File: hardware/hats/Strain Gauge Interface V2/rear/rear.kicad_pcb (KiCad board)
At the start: 2 copper layers, 78 x 58 mm, 76 parts, among them J1 Conn_01x14, U1 ADS1235IRHBT, U2 ADS1235IRHBT, U3 LMR50410YQDBVRQ1, U5 BD450, U6 BD433

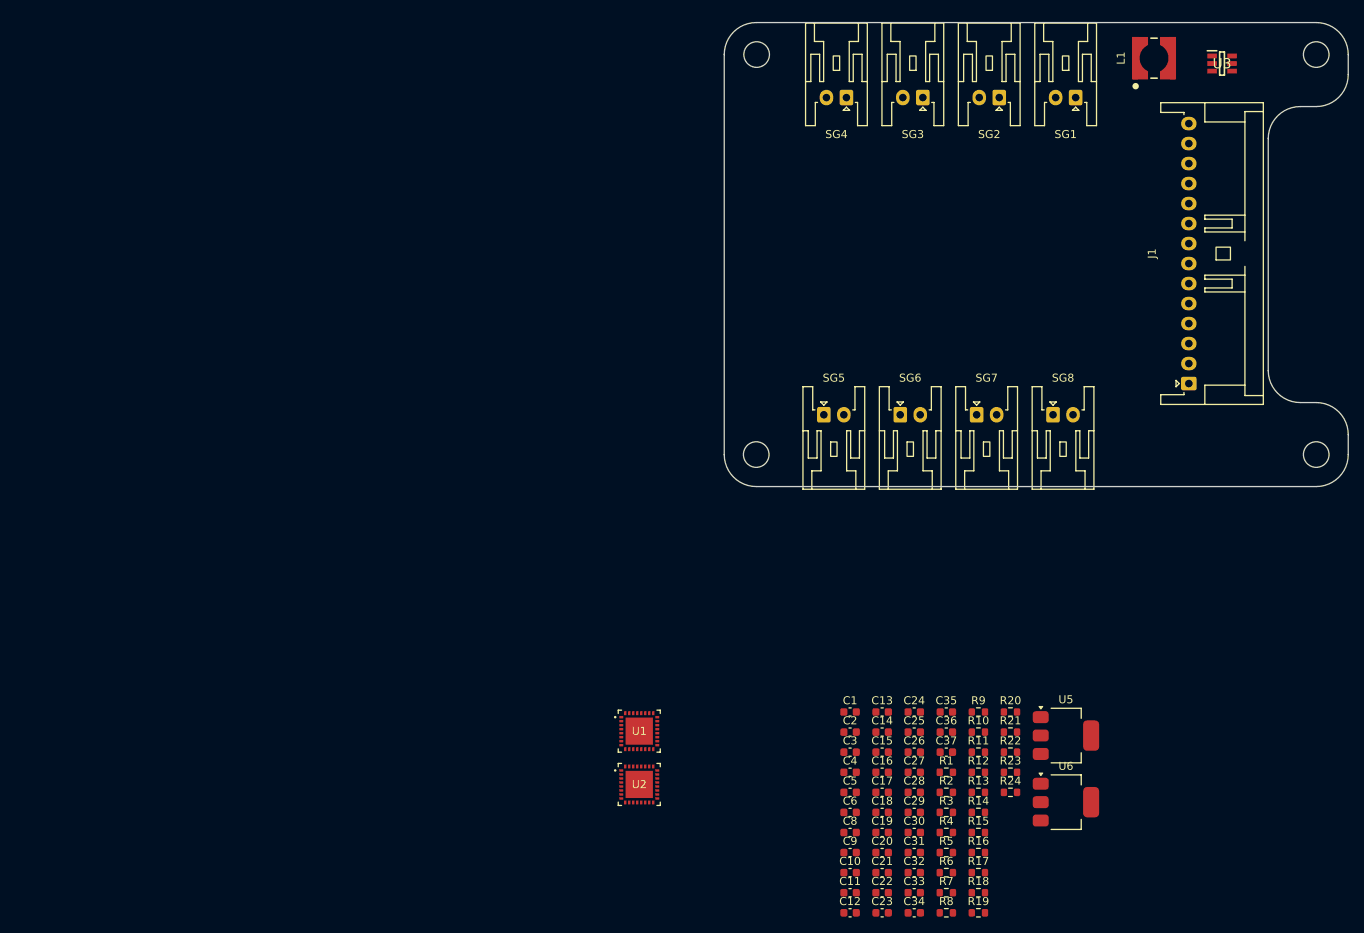
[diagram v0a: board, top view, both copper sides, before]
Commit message: this is worse than torture
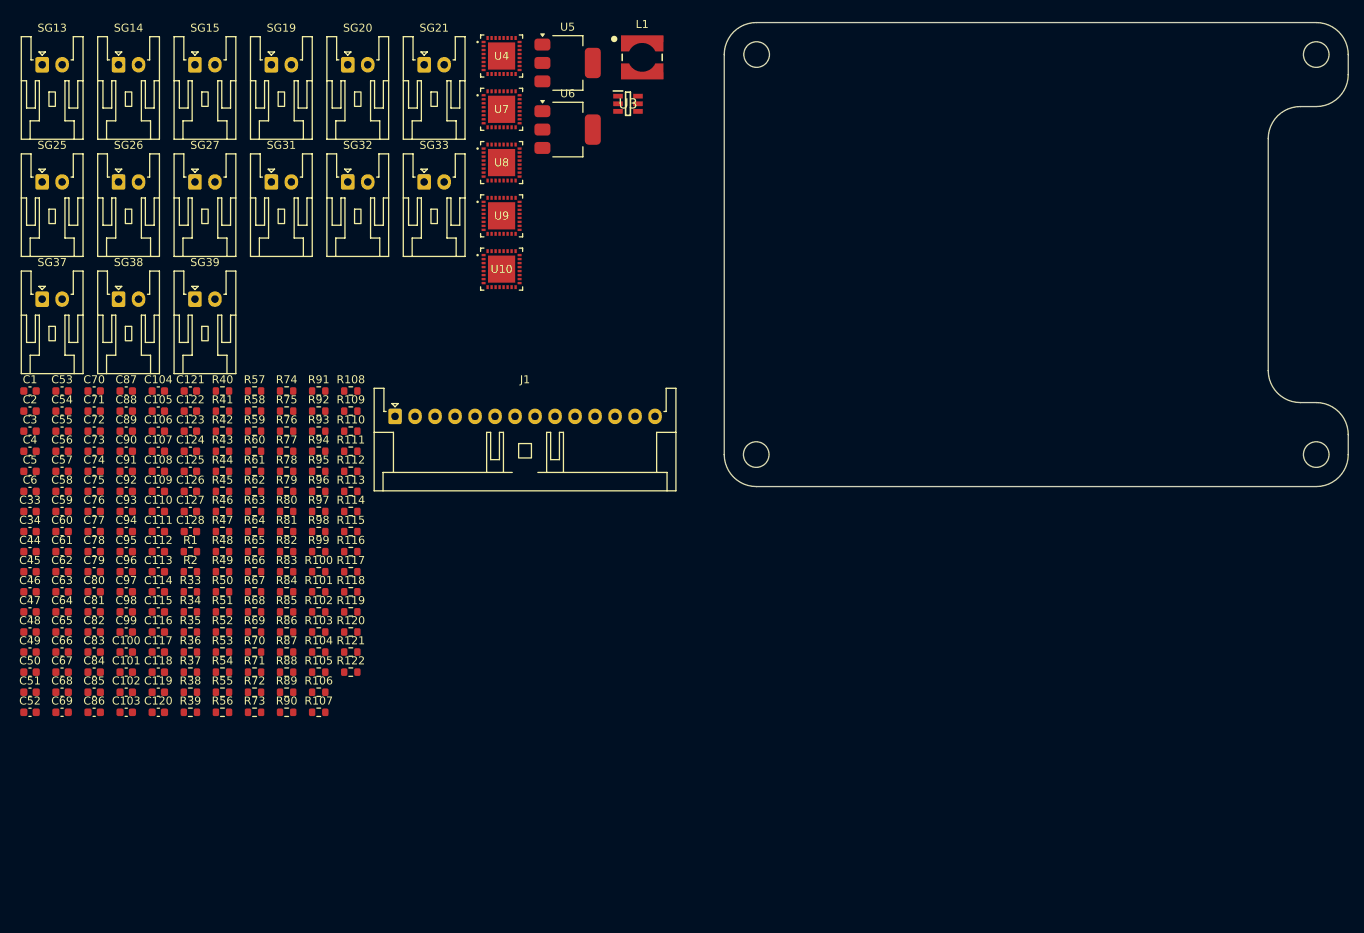
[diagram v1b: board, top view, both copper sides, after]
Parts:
- removed C10, C11, C12, C13, C14, C15, C17, C8: 1uf, Capacitor_SMD:C_0603_1608Metric
- removed C16, C18, C21, C26, C29, C32, C37, C9: 10nf, Capacitor_SMD:C_0603_1608Metric
- removed C19, C20, C22, C23, C24, C25, C27, C28, C30, C31, C35, C36: 1nf, Capacitor_SMD:C_0603_1608Metric
- removed R10, R11, R14, R15, R18, R19, R23, R24, R6, R7, R8, R9: 100, Resistor_SMD:R_0603_1608Metric
- removed R12, R13, R16, R17, R20, R21, R3, R5: 120, Resistor_SMD:R_0603_1608Metric
- removed R22, R4: 100k, Resistor_SMD:R_0603_1608Metric
- removed SG1, SG3, SG5, SG7: TOP, Connector_JST:JST_XA_S02B-XASK-1_1x02_P2.50mm_Horizontal
- removed SG2, SG4, SG6, SG8: BOTTOM, Connector_JST:JST_XA_S02B-XASK-1_1x02_P2.50mm_Horizontal
- removed U1, U2: ADS1235IRHBT, CustomFootprints:RHB32_TEX
- added C100: 1nf, Capacitor_SMD:C_0603_1608Metric, F.Cu at (32.2, 136.1)
- added C101: 10nf, Capacitor_SMD:C_0603_1608Metric, F.Cu at (32.2, 138.6)
- added C102: 10nf, Capacitor_SMD:C_0603_1608Metric, F.Cu at (32.2, 141.1)
- added C103: 10nf, Capacitor_SMD:C_0603_1608Metric, F.Cu at (32.2, 143.6)
- added C104: 1nf, Capacitor_SMD:C_0603_1608Metric, F.Cu at (36.3, 103.4)
- added C105: 1nf, Capacitor_SMD:C_0603_1608Metric, F.Cu at (36.3, 105.9)
- added C106: 1nf, Capacitor_SMD:C_0603_1608Metric, F.Cu at (36.3, 108.5)
- added C107: 1nf, Capacitor_SMD:C_0603_1608Metric, F.Cu at (36.3, 111.0)
- added C108: 1nf, Capacitor_SMD:C_0603_1608Metric, F.Cu at (36.3, 113.5)
- added C109: 1nf, Capacitor_SMD:C_0603_1608Metric, F.Cu at (36.3, 116.0)
- added C110: 10nf, Capacitor_SMD:C_0603_1608Metric, F.Cu at (36.3, 118.5)
- added C111: 10nf, Capacitor_SMD:C_0603_1608Metric, F.Cu at (36.3, 121.0)
- added C112: 10nf, Capacitor_SMD:C_0603_1608Metric, F.Cu at (36.3, 123.5)
- added C113: 1uf, Capacitor_SMD:C_0603_1608Metric, F.Cu at (36.3, 126.0)
- added C114: 1uf, Capacitor_SMD:C_0603_1608Metric, F.Cu at (36.3, 128.5)
- added C115: 1uf, Capacitor_SMD:C_0603_1608Metric, F.Cu at (36.3, 131.0)
- added C116: 10nf, Capacitor_SMD:C_0603_1608Metric, F.Cu at (36.3, 133.6)
- added C117: 1uf, Capacitor_SMD:C_0603_1608Metric, F.Cu at (36.3, 136.1)
- added C118: 1nf, Capacitor_SMD:C_0603_1608Metric, F.Cu at (36.3, 138.6)
- added C119: 1nf, Capacitor_SMD:C_0603_1608Metric, F.Cu at (36.3, 141.1)
- added C120: 10nf, Capacitor_SMD:C_0603_1608Metric, F.Cu at (36.3, 143.6)
- added C121: 1uf, Capacitor_SMD:C_0603_1608Metric, F.Cu at (40.3, 103.4)
- added C122: 1uf, Capacitor_SMD:C_0603_1608Metric, F.Cu at (40.3, 105.9)
- added C123: 1uf, Capacitor_SMD:C_0603_1608Metric, F.Cu at (40.3, 108.5)
- added C124: 10nf, Capacitor_SMD:C_0603_1608Metric, F.Cu at (40.3, 111.0)
- added C125: 1uf, Capacitor_SMD:C_0603_1608Metric, F.Cu at (40.3, 113.5)
- added C126: 1nf, Capacitor_SMD:C_0603_1608Metric, F.Cu at (40.3, 116.0)
- added C127: 1nf, Capacitor_SMD:C_0603_1608Metric, F.Cu at (40.3, 118.5)
- added C128: 10nf, Capacitor_SMD:C_0603_1608Metric, F.Cu at (40.3, 121.0)
- added C44: 1uf, Capacitor_SMD:C_0603_1608Metric, F.Cu at (20.2, 123.5)
- added C45: 1uf, Capacitor_SMD:C_0603_1608Metric, F.Cu at (20.2, 126.0)
- added C46: 1uf, Capacitor_SMD:C_0603_1608Metric, F.Cu at (20.2, 128.5)
- added C47: 1uf, Capacitor_SMD:C_0603_1608Metric, F.Cu at (20.2, 131.0)
- added C48: 1uf, Capacitor_SMD:C_0603_1608Metric, F.Cu at (20.2, 133.6)
- added C49: 1uf, Capacitor_SMD:C_0603_1608Metric, F.Cu at (20.2, 136.1)
- added C50: 10nf, Capacitor_SMD:C_0603_1608Metric, F.Cu at (20.2, 138.6)
- added C51: 10nf, Capacitor_SMD:C_0603_1608Metric, F.Cu at (20.2, 141.1)
- added C52: 1uf, Capacitor_SMD:C_0603_1608Metric, F.Cu at (20.2, 143.6)
- added C53: 1uf, Capacitor_SMD:C_0603_1608Metric, F.Cu at (24.2, 103.4)
- added C54: 1nf, Capacitor_SMD:C_0603_1608Metric, F.Cu at (24.2, 105.9)
- added C55: 1nf, Capacitor_SMD:C_0603_1608Metric, F.Cu at (24.2, 108.5)
- added C56: 1nf, Capacitor_SMD:C_0603_1608Metric, F.Cu at (24.2, 111.0)
- added C57: 1nf, Capacitor_SMD:C_0603_1608Metric, F.Cu at (24.2, 113.5)
- added C58: 10nf, Capacitor_SMD:C_0603_1608Metric, F.Cu at (24.2, 116.0)
- added C59: 10nf, Capacitor_SMD:C_0603_1608Metric, F.Cu at (24.2, 118.5)
- added C60: 1uf, Capacitor_SMD:C_0603_1608Metric, F.Cu at (24.2, 121.0)
- added C61: 1uf, Capacitor_SMD:C_0603_1608Metric, F.Cu at (24.2, 123.5)
- added C62: 1uf, Capacitor_SMD:C_0603_1608Metric, F.Cu at (24.2, 126.0)
- added C63: 10nf, Capacitor_SMD:C_0603_1608Metric, F.Cu at (24.2, 128.5)
- added C64: 1uf, Capacitor_SMD:C_0603_1608Metric, F.Cu at (24.2, 131.0)
- added C65: 1nf, Capacitor_SMD:C_0603_1608Metric, F.Cu at (24.2, 133.6)
- added C66: 1nf, Capacitor_SMD:C_0603_1608Metric, F.Cu at (24.2, 136.1)
- added C67: 10nf, Capacitor_SMD:C_0603_1608Metric, F.Cu at (24.2, 138.6)
- added C68: 1nf, Capacitor_SMD:C_0603_1608Metric, F.Cu at (24.2, 141.1)
- added C69: 1nf, Capacitor_SMD:C_0603_1608Metric, F.Cu at (24.2, 143.6)
- added C70: 1nf, Capacitor_SMD:C_0603_1608Metric, F.Cu at (28.2, 103.4)
- added C71: 1nf, Capacitor_SMD:C_0603_1608Metric, F.Cu at (28.2, 105.9)
- added C72: 1nf, Capacitor_SMD:C_0603_1608Metric, F.Cu at (28.2, 108.5)
- added C73: 1nf, Capacitor_SMD:C_0603_1608Metric, F.Cu at (28.2, 111.0)
- added C74: 10nf, Capacitor_SMD:C_0603_1608Metric, F.Cu at (28.2, 113.5)
- added C75: 10nf, Capacitor_SMD:C_0603_1608Metric, F.Cu at (28.2, 116.0)
- added C76: 10nf, Capacitor_SMD:C_0603_1608Metric, F.Cu at (28.2, 118.5)
- added C77: 1nf, Capacitor_SMD:C_0603_1608Metric, F.Cu at (28.2, 121.0)
- added C78: 1nf, Capacitor_SMD:C_0603_1608Metric, F.Cu at (28.2, 123.5)
- added C79: 1nf, Capacitor_SMD:C_0603_1608Metric, F.Cu at (28.2, 126.0)
- added C80: 1nf, Capacitor_SMD:C_0603_1608Metric, F.Cu at (28.2, 128.5)
- added C81: 1nf, Capacitor_SMD:C_0603_1608Metric, F.Cu at (28.2, 131.0)
- added C82: 1nf, Capacitor_SMD:C_0603_1608Metric, F.Cu at (28.2, 133.6)
- added C83: 10nf, Capacitor_SMD:C_0603_1608Metric, F.Cu at (28.2, 136.1)
- added C84: 10nf, Capacitor_SMD:C_0603_1608Metric, F.Cu at (28.2, 138.6)
- added C85: 10nf, Capacitor_SMD:C_0603_1608Metric, F.Cu at (28.2, 141.1)
- added C86: 1nf, Capacitor_SMD:C_0603_1608Metric, F.Cu at (28.2, 143.6)
- added C87: 1nf, Capacitor_SMD:C_0603_1608Metric, F.Cu at (32.2, 103.4)
- added C88: 1nf, Capacitor_SMD:C_0603_1608Metric, F.Cu at (32.2, 105.9)
- added C89: 1nf, Capacitor_SMD:C_0603_1608Metric, F.Cu at (32.2, 108.5)
- added C90: 1nf, Capacitor_SMD:C_0603_1608Metric, F.Cu at (32.2, 111.0)
- added C91: 1nf, Capacitor_SMD:C_0603_1608Metric, F.Cu at (32.2, 113.5)
- added C92: 10nf, Capacitor_SMD:C_0603_1608Metric, F.Cu at (32.2, 116.0)
- added C93: 10nf, Capacitor_SMD:C_0603_1608Metric, F.Cu at (32.2, 118.5)
- added C94: 10nf, Capacitor_SMD:C_0603_1608Metric, F.Cu at (32.2, 121.0)
- added C95: 1nf, Capacitor_SMD:C_0603_1608Metric, F.Cu at (32.2, 123.5)
- added C96: 1nf, Capacitor_SMD:C_0603_1608Metric, F.Cu at (32.2, 126.0)
- added C97: 1nf, Capacitor_SMD:C_0603_1608Metric, F.Cu at (32.2, 128.5)
- added C98: 1nf, Capacitor_SMD:C_0603_1608Metric, F.Cu at (32.2, 131.0)
- added C99: 1nf, Capacitor_SMD:C_0603_1608Metric, F.Cu at (32.2, 133.6)
- added R100: 120, Resistor_SMD:R_0603_1608Metric, F.Cu at (56.3, 126.0)
- added R101: 120, Resistor_SMD:R_0603_1608Metric, F.Cu at (56.3, 128.5)
- added R102: 120, Resistor_SMD:R_0603_1608Metric, F.Cu at (56.3, 131.0)
- added R103: 120, Resistor_SMD:R_0603_1608Metric, F.Cu at (56.3, 133.6)
- added R104: 120, Resistor_SMD:R_0603_1608Metric, F.Cu at (56.3, 136.1)
- added R105: 120, Resistor_SMD:R_0603_1608Metric, F.Cu at (56.3, 138.6)
- added R106: 120, Resistor_SMD:R_0603_1608Metric, F.Cu at (56.3, 141.1)
- added R107: 120, Resistor_SMD:R_0603_1608Metric, F.Cu at (56.3, 143.6)
- added R108: 120, Resistor_SMD:R_0603_1608Metric, F.Cu at (60.3, 103.4)
- added R109: 120, Resistor_SMD:R_0603_1608Metric, F.Cu at (60.3, 105.9)
- added R110: 120, Resistor_SMD:R_0603_1608Metric, F.Cu at (60.3, 108.5)
- added R111: 120, Resistor_SMD:R_0603_1608Metric, F.Cu at (60.3, 111.0)
- added R112: 120, Resistor_SMD:R_0603_1608Metric, F.Cu at (60.3, 113.5)
- added R113: 120, Resistor_SMD:R_0603_1608Metric, F.Cu at (60.3, 116.0)
- added R114: 120, Resistor_SMD:R_0603_1608Metric, F.Cu at (60.3, 118.5)
- added R115: 120, Resistor_SMD:R_0603_1608Metric, F.Cu at (60.3, 121.0)
- added R116: 120, Resistor_SMD:R_0603_1608Metric, F.Cu at (60.3, 123.5)
- added R117: 100k, Resistor_SMD:R_0603_1608Metric, F.Cu at (60.3, 126.0)
- added R118: 100, Resistor_SMD:R_0603_1608Metric, F.Cu at (60.3, 128.5)
- added R119: 100, Resistor_SMD:R_0603_1608Metric, F.Cu at (60.3, 131.0)
- added R120: 100k, Resistor_SMD:R_0603_1608Metric, F.Cu at (60.3, 133.6)
- added R121: 100, Resistor_SMD:R_0603_1608Metric, F.Cu at (60.3, 136.1)
- added R122: 100, Resistor_SMD:R_0603_1608Metric, F.Cu at (60.3, 138.6)
- added R33: 100k, Resistor_SMD:R_0603_1608Metric, F.Cu at (40.3, 128.5)
- added R34: 100k, Resistor_SMD:R_0603_1608Metric, F.Cu at (40.3, 131.0)
- added R35: 100, Resistor_SMD:R_0603_1608Metric, F.Cu at (40.3, 133.6)
- added R36: 100, Resistor_SMD:R_0603_1608Metric, F.Cu at (40.3, 136.1)
- added R37: 100, Resistor_SMD:R_0603_1608Metric, F.Cu at (40.3, 138.6)
- added R38: 100, Resistor_SMD:R_0603_1608Metric, F.Cu at (40.3, 141.1)
- added R39: 100k, Resistor_SMD:R_0603_1608Metric, F.Cu at (40.3, 143.6)
- added R40: 100, Resistor_SMD:R_0603_1608Metric, F.Cu at (44.3, 103.4)
- added R41: 100, Resistor_SMD:R_0603_1608Metric, F.Cu at (44.3, 105.9)
- added R42: 100, Resistor_SMD:R_0603_1608Metric, F.Cu at (44.3, 108.5)
- added R43: 100, Resistor_SMD:R_0603_1608Metric, F.Cu at (44.3, 111.0)
- added R44: 100, Resistor_SMD:R_0603_1608Metric, F.Cu at (44.3, 113.5)
- added R45: 100, Resistor_SMD:R_0603_1608Metric, F.Cu at (44.3, 116.0)
- added R46: 100, Resistor_SMD:R_0603_1608Metric, F.Cu at (44.3, 118.5)
- added R47: 100, Resistor_SMD:R_0603_1608Metric, F.Cu at (44.3, 121.0)
- added R48: 120, Resistor_SMD:R_0603_1608Metric, F.Cu at (44.3, 123.5)
- added R49: 120, Resistor_SMD:R_0603_1608Metric, F.Cu at (44.3, 126.0)
- added R50: 120, Resistor_SMD:R_0603_1608Metric, F.Cu at (44.3, 128.5)
- added R51: 120, Resistor_SMD:R_0603_1608Metric, F.Cu at (44.3, 131.0)
- added R52: 120, Resistor_SMD:R_0603_1608Metric, F.Cu at (44.3, 133.6)
- added R53: 120, Resistor_SMD:R_0603_1608Metric, F.Cu at (44.3, 136.1)
- added R54: 100, Resistor_SMD:R_0603_1608Metric, F.Cu at (44.3, 138.6)
- added R55: 100, Resistor_SMD:R_0603_1608Metric, F.Cu at (44.3, 141.1)
- added R56: 100, Resistor_SMD:R_0603_1608Metric, F.Cu at (44.3, 143.6)
- added R57: 100, Resistor_SMD:R_0603_1608Metric, F.Cu at (48.3, 103.4)
- added R58: 100, Resistor_SMD:R_0603_1608Metric, F.Cu at (48.3, 105.9)
- added R59: 100, Resistor_SMD:R_0603_1608Metric, F.Cu at (48.3, 108.5)
- added R60: 120, Resistor_SMD:R_0603_1608Metric, F.Cu at (48.3, 111.0)
- added R61: 120, Resistor_SMD:R_0603_1608Metric, F.Cu at (48.3, 113.5)
- added R62: 120, Resistor_SMD:R_0603_1608Metric, F.Cu at (48.3, 116.0)
- added R63: 120, Resistor_SMD:R_0603_1608Metric, F.Cu at (48.3, 118.5)
- added R64: 120, Resistor_SMD:R_0603_1608Metric, F.Cu at (48.3, 121.0)
- added R65: 120, Resistor_SMD:R_0603_1608Metric, F.Cu at (48.3, 123.5)
- added R66: 100, Resistor_SMD:R_0603_1608Metric, F.Cu at (48.3, 126.0)
- added R67: 100, Resistor_SMD:R_0603_1608Metric, F.Cu at (48.3, 128.5)
- added R68: 100, Resistor_SMD:R_0603_1608Metric, F.Cu at (48.3, 131.0)
- added R69: 100, Resistor_SMD:R_0603_1608Metric, F.Cu at (48.3, 133.6)
- added R70: 100, Resistor_SMD:R_0603_1608Metric, F.Cu at (48.3, 136.1)
- added R71: 100, Resistor_SMD:R_0603_1608Metric, F.Cu at (48.3, 138.6)
- added R72: 120, Resistor_SMD:R_0603_1608Metric, F.Cu at (48.3, 141.1)
- added R73: 120, Resistor_SMD:R_0603_1608Metric, F.Cu at (48.3, 143.6)
- added R74: 120, Resistor_SMD:R_0603_1608Metric, F.Cu at (52.3, 103.4)
- added R75: 120, Resistor_SMD:R_0603_1608Metric, F.Cu at (52.3, 105.9)
- added R76: 120, Resistor_SMD:R_0603_1608Metric, F.Cu at (52.3, 108.5)
- added R77: 120, Resistor_SMD:R_0603_1608Metric, F.Cu at (52.3, 111.0)
- added R78: 100, Resistor_SMD:R_0603_1608Metric, F.Cu at (52.3, 113.5)
- added R79: 100, Resistor_SMD:R_0603_1608Metric, F.Cu at (52.3, 116.0)
- added R80: 100, Resistor_SMD:R_0603_1608Metric, F.Cu at (52.3, 118.5)
- added R81: 100, Resistor_SMD:R_0603_1608Metric, F.Cu at (52.3, 121.0)
- added R82: 100, Resistor_SMD:R_0603_1608Metric, F.Cu at (52.3, 123.5)
- added R83: 100, Resistor_SMD:R_0603_1608Metric, F.Cu at (52.3, 126.0)
- added R84: 120, Resistor_SMD:R_0603_1608Metric, F.Cu at (52.3, 128.5)
- added R85: 120, Resistor_SMD:R_0603_1608Metric, F.Cu at (52.3, 131.0)
- added R86: 120, Resistor_SMD:R_0603_1608Metric, F.Cu at (52.3, 133.6)
- added R87: 120, Resistor_SMD:R_0603_1608Metric, F.Cu at (52.3, 136.1)
- added R88: 120, Resistor_SMD:R_0603_1608Metric, F.Cu at (52.3, 138.6)
- added R89: 120, Resistor_SMD:R_0603_1608Metric, F.Cu at (52.3, 141.1)
- added R90: 100, Resistor_SMD:R_0603_1608Metric, F.Cu at (52.3, 143.6)
- added R91: 100, Resistor_SMD:R_0603_1608Metric, F.Cu at (56.3, 103.4)
- added R92: 100, Resistor_SMD:R_0603_1608Metric, F.Cu at (56.3, 105.9)
- added R93: 100, Resistor_SMD:R_0603_1608Metric, F.Cu at (56.3, 108.5)
- added R94: 100, Resistor_SMD:R_0603_1608Metric, F.Cu at (56.3, 111.0)
- added R95: 100, Resistor_SMD:R_0603_1608Metric, F.Cu at (56.3, 113.5)
- added R96: 120, Resistor_SMD:R_0603_1608Metric, F.Cu at (56.3, 116.0)
- added R97: 120, Resistor_SMD:R_0603_1608Metric, F.Cu at (56.3, 118.5)
- added R98: 120, Resistor_SMD:R_0603_1608Metric, F.Cu at (56.3, 121.0)
- added R99: 120, Resistor_SMD:R_0603_1608Metric, F.Cu at (56.3, 123.5)
- added SG13: 45D, Connector_JST:JST_XA_S02B-XASK-1_1x02_P2.50mm_Horizontal, F.Cu at (21.7, 62.6)
- added SG14: 90D, Connector_JST:JST_XA_S02B-XASK-1_1x02_P2.50mm_Horizontal, F.Cu at (31.3, 62.6)
- added SG15: 0D, Connector_JST:JST_XA_S02B-XASK-1_1x02_P2.50mm_Horizontal, F.Cu at (40.8, 62.6)
- added SG19: 45D, Connector_JST:JST_XA_S02B-XASK-1_1x02_P2.50mm_Horizontal, F.Cu at (50.4, 62.6)
- added SG20: 90D, Connector_JST:JST_XA_S02B-XASK-1_1x02_P2.50mm_Horizontal, F.Cu at (59.9, 62.6)
- added SG21: 0D, Connector_JST:JST_XA_S02B-XASK-1_1x02_P2.50mm_Horizontal, F.Cu at (69.5, 62.6)
- added SG25: 45D, Connector_JST:JST_XA_S02B-XASK-1_1x02_P2.50mm_Horizontal, F.Cu at (21.7, 77.3)
- added SG26: 90D, Connector_JST:JST_XA_S02B-XASK-1_1x02_P2.50mm_Horizontal, F.Cu at (31.3, 77.3)
- added SG27: 0D, Connector_JST:JST_XA_S02B-XASK-1_1x02_P2.50mm_Horizontal, F.Cu at (40.8, 77.3)
- added SG31: 45D, Connector_JST:JST_XA_S02B-XASK-1_1x02_P2.50mm_Horizontal, F.Cu at (50.4, 77.3)
- added SG32: 90D, Connector_JST:JST_XA_S02B-XASK-1_1x02_P2.50mm_Horizontal, F.Cu at (59.9, 77.3)
- added SG33: 0D, Connector_JST:JST_XA_S02B-XASK-1_1x02_P2.50mm_Horizontal, F.Cu at (69.5, 77.3)
- added SG37: 45D, Connector_JST:JST_XA_S02B-XASK-1_1x02_P2.50mm_Horizontal, F.Cu at (21.7, 92.0)
- added SG38: 90D, Connector_JST:JST_XA_S02B-XASK-1_1x02_P2.50mm_Horizontal, F.Cu at (31.3, 92.0)
- added SG39: 0D, Connector_JST:JST_XA_S02B-XASK-1_1x02_P2.50mm_Horizontal, F.Cu at (40.8, 92.0)
- added U10: ADS1235IRHBT, CustomFootprints:RHB32_TEX, F.Cu at (79.2, 88.2)
- added U4: ADS1235IRHBT, CustomFootprints:RHB32_TEX, F.Cu at (79.2, 61.6)
- added U7: ADS1235IRHBT, CustomFootprints:RHB32_TEX, F.Cu at (79.2, 68.2)
- added U8: ADS1235IRHBT, CustomFootprints:RHB32_TEX, F.Cu at (79.2, 74.9)
- added U9: ADS1235IRHBT, CustomFootprints:RHB32_TEX, F.Cu at (79.2, 81.5)
- moved C33 120.4 mm to (20.2, 118.5)
- moved C34 120.4 mm to (20.2, 121.0)
- moved C1 110.1 mm to (20.2, 103.4)
- moved C2 110.1 mm to (20.2, 105.9)
- moved C3 110.1 mm to (20.2, 108.5)
- moved C4 110.1 mm to (20.2, 111.0)
- moved C5 110.1 mm to (20.2, 113.5)
- moved C6 110.1 mm to (20.2, 116.0)
- moved U5 104.6 mm to (87.4, 62.4)
- moved U6 104.6 mm to (87.4, 70.8)
- moved J1 99.3 mm to (65.8, 106.6), turned to 0 degrees
- moved R1 98.4 mm to (40.3, 123.5)
- moved R2 98.4 mm to (40.3, 126.0)
- moved U3 74.4 mm to (95.0, 67.5)
- moved L1 64.0 mm to (96.7, 61.7), turned to 0 degrees
